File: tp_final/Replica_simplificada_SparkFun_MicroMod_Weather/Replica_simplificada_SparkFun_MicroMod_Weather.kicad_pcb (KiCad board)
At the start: 2 copper layers, 40.1 x 40.1 mm, 40 parts, among them J1 USB_C_Receptacle_USB2.0, J2 Conn_01x05, J3 Conn_01x02, J4 Conn_01x03, U1 BME280, U2 AP7361C-33F, U3 AS3935

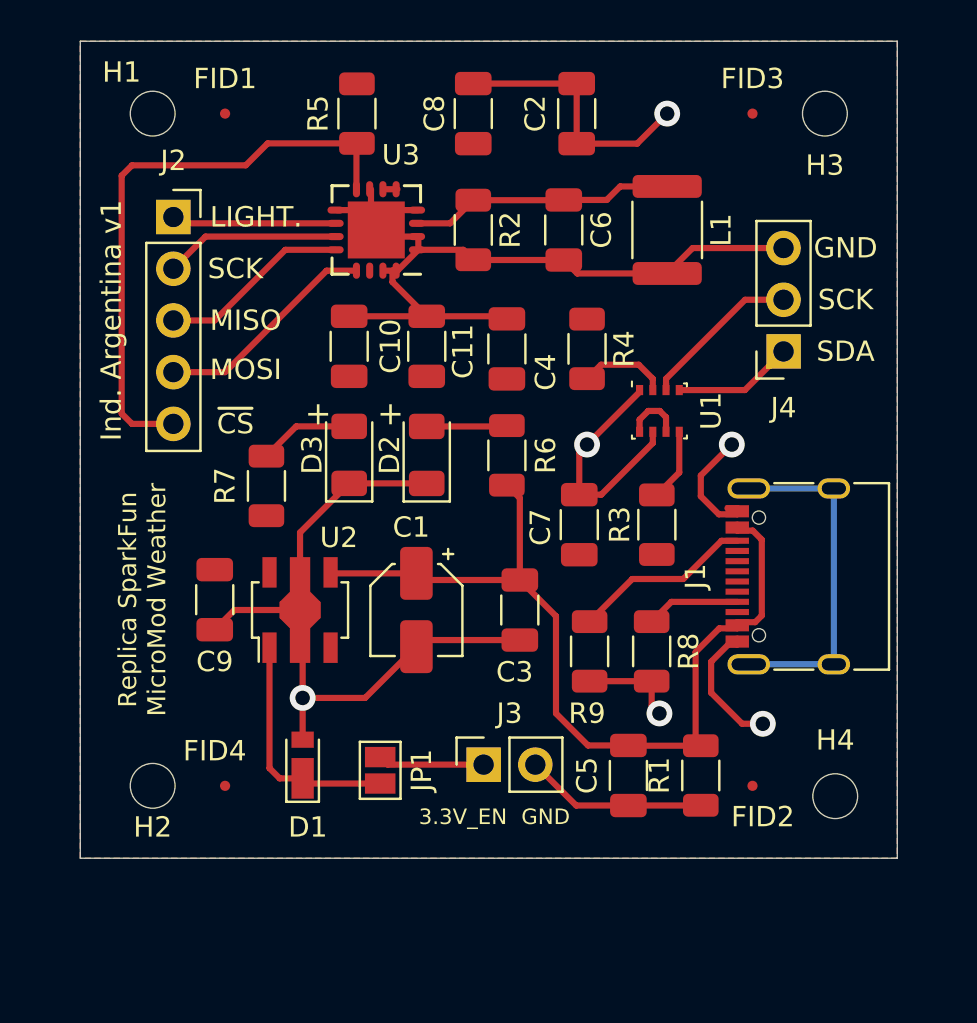
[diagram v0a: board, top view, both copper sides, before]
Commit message: Correciones finales
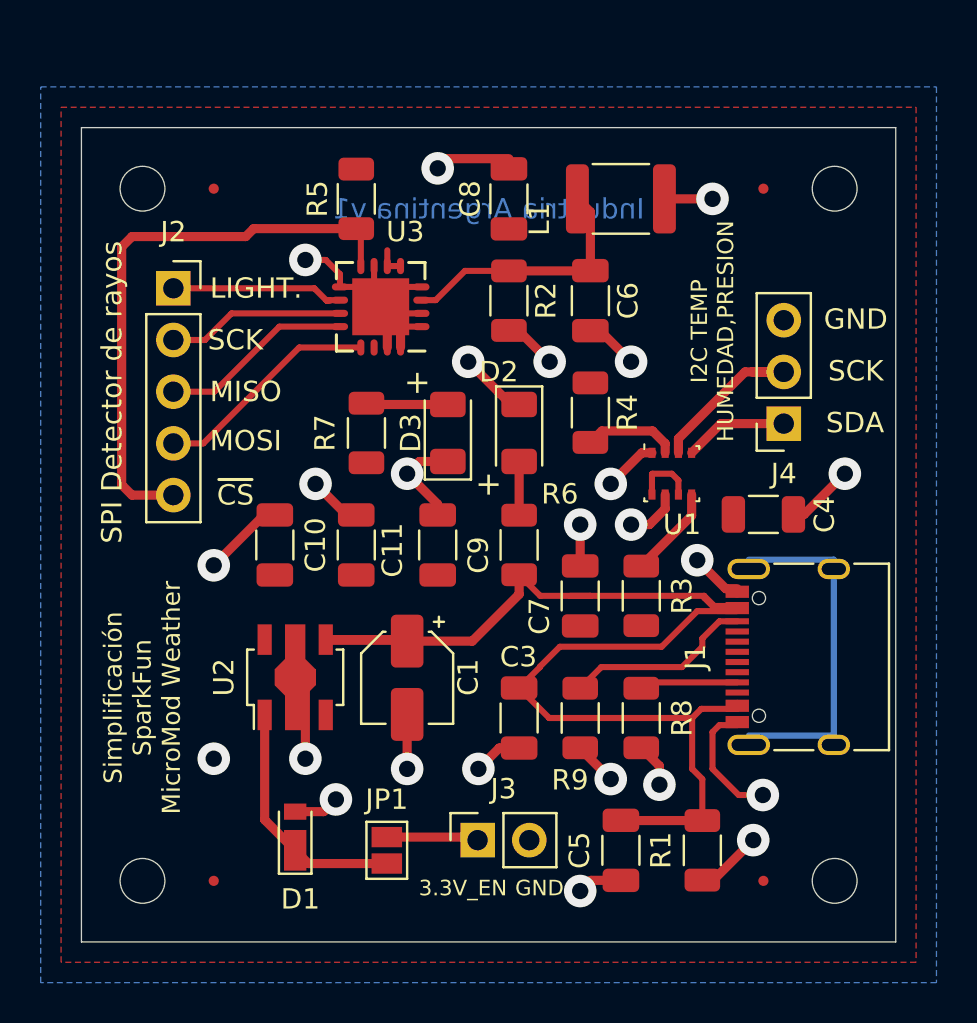
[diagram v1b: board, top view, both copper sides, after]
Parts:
- removed C2: 10u, Capacitor_SMD:C_1206_3216Metric
- C1, C9: value 10u -> 10uF
- C10, C8: value 1u -> 1uF
- C11, C3: value 0.22u -> 0.22uF
- C4, C7: value 0.1u -> 0.1uF
- C6: value 1n -> 1nC
- L1: value 100u -> 100uH
- moved C4 15.0 mm to (157.0, 103.0), turned to 0 degrees
- moved C9 11.3 mm to (141.0, 104.5), turned to 90 degrees
- moved C10 10.4 mm to (133.0, 104.5)
- moved C11 10.4 mm to (137.0, 104.5)
- moved R7 5.56 mm to (137.5, 99.0)
- moved C3 5.30 mm to (145.0, 113.0)
- moved D3 4.97 mm to (141.5, 99.0)
- moved FID4 4.70 mm to (130.0, 121.0)
- moved FID2 4.70 mm to (157.0, 121.0)
- moved H2 4.69 mm to (126.5, 121.0)
- moved D2 4.66 mm to (145.0, 99.0), turned to 270 degrees
- moved C8 4.54 mm to (144.5, 87.5)
- moved R6 4.44 mm to (145.0, 104.5)
- moved R5 4.19 mm to (137.0, 87.5)
- moved H4 4.16 mm to (160.5, 121.0)
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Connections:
- net 3.3V_EN renamed /3.3V_EN
- net I2C_SCK renamed /I2C_SCK
- net I2C_SDA renamed /I2C_SDA
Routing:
- net GND: track 127.0 -> 86.6 mm, vias 6 -> 24
- net +5V: track 43.5 -> 63.2 mm
- net Net-(D2-Pad2): track 3.95 -> 2.64 mm
- net +3V3: track 3.57 -> 4.57 mm
- net Net-(R3-Pad2): track 3.56 -> 4.54 mm
- net /I2C_SCK: track 5.91 -> 5.12 mm
- net /3.3V_EN: track 5.27 -> 4.52 mm
- net /SPI_~CS~: track 28.9 -> 28.3 mm
- net Net-(D3-Pad2): track 4.67 -> 4.03 mm
- net /I2C_SDA: track 8.26 -> 8.80 mm
- net /LIGHTING_IRQ: track 8.10 -> 8.62 mm
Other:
- board size 40.1 x 40.1 mm -> 40 x 40 mm
- net class Default: clearance 0.1524 -> 0.2; trace_width 0.3048 -> 0.3; via_drill 0.7112 -> 0.7
- rule trace_clearance: 0.1524 -> 0.2
- rule trace_min: 0.127 -> 0.3
- rule via_min_drill: 0.5 -> 0.7
- rule via_min_size: 1.1096 -> 1.27
- board text added: "I2C TEMP HUMEDAD,PRESION"
- board text added: "Industria Argentina v1"
- board text added: "Minimos en base a fabricante Mayer PCB (12 mils) Margen: 1mm Grillas: 1mm, 0.5mm Minimo ancho de pista: 0.3mm Diametro de via: 1.27 mm Diametro de agujero: 0.7 mm Terminación: HASL"
- board text added: "SPI Detector de rayos"
- board text added: "Simplificación SparkFun MicroMod Weather"
- board text removed: "Ind. Argentina v1"
- board text removed: "Margen: 6 mils Grilla: 20 mils"
- board text removed: "Minimo ancho de pista: 5 mils Minimo diamtero via: 1.1 mm Minimo taladro: 0.5 mm"
- board text removed: "Replica SparkFun MicroMod Weather"
- board text removed: "Valores tomados en base a fabricante: Mayer PCB"
